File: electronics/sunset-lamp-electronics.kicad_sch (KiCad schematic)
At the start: 32 parts, among them J1 Screw_Terminal_01x02, J2 Screw_Terminal_01x02, J3 Conn_01x12_Male, J4 Conn_01x08_Male, J5 Conn_02x03_Counter_Clockwise, Q1 IRL3705N, SW1 SW_Push, U1 LM78M05CDTX/NOPB, U2 DS1307Z+T&R, U3 ATMEGA328P-AU, Y1 AB38T-32.768KHZ

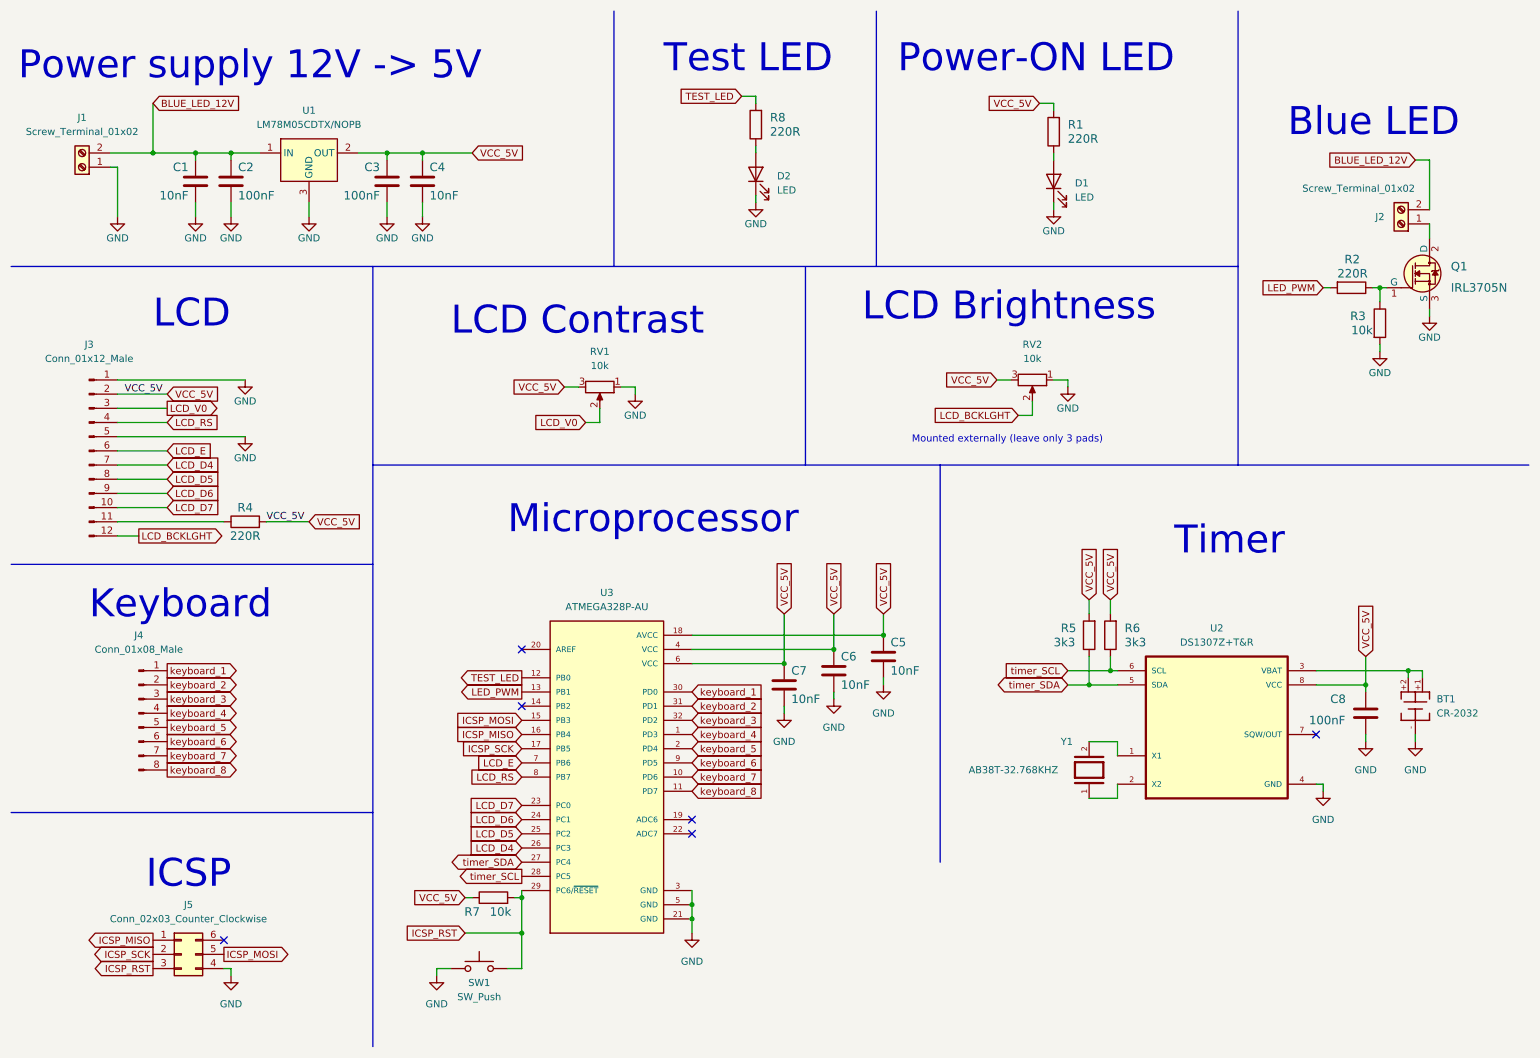
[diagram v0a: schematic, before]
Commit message: Commit before local repo deletion
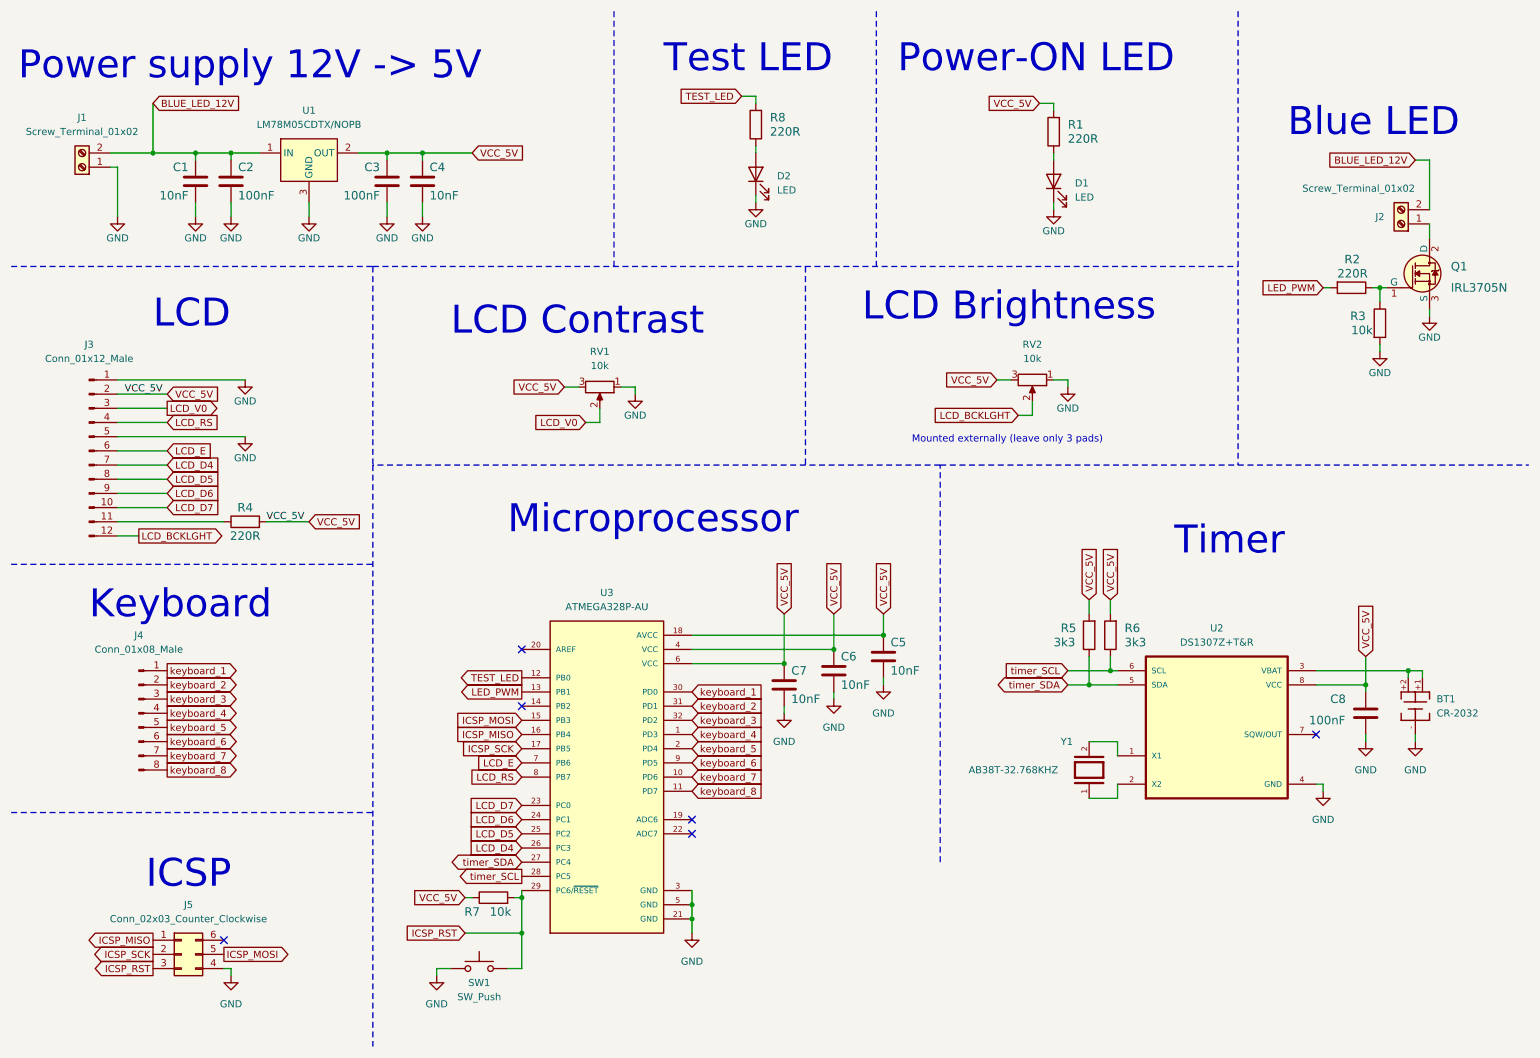
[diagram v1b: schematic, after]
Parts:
- U1: symbol iridiumLinearVoltageRegulators:LM78M05CDTX/NOPB -> iridiumLinearVoltageRegulators:LM78M05CDTX/NOPB
